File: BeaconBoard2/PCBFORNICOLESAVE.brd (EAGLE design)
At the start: 101.6 x 101.6 mm, 104 parts, among them Q3 FDN340P, U1 ATMega2560, U2 3X3BGA0.4MM

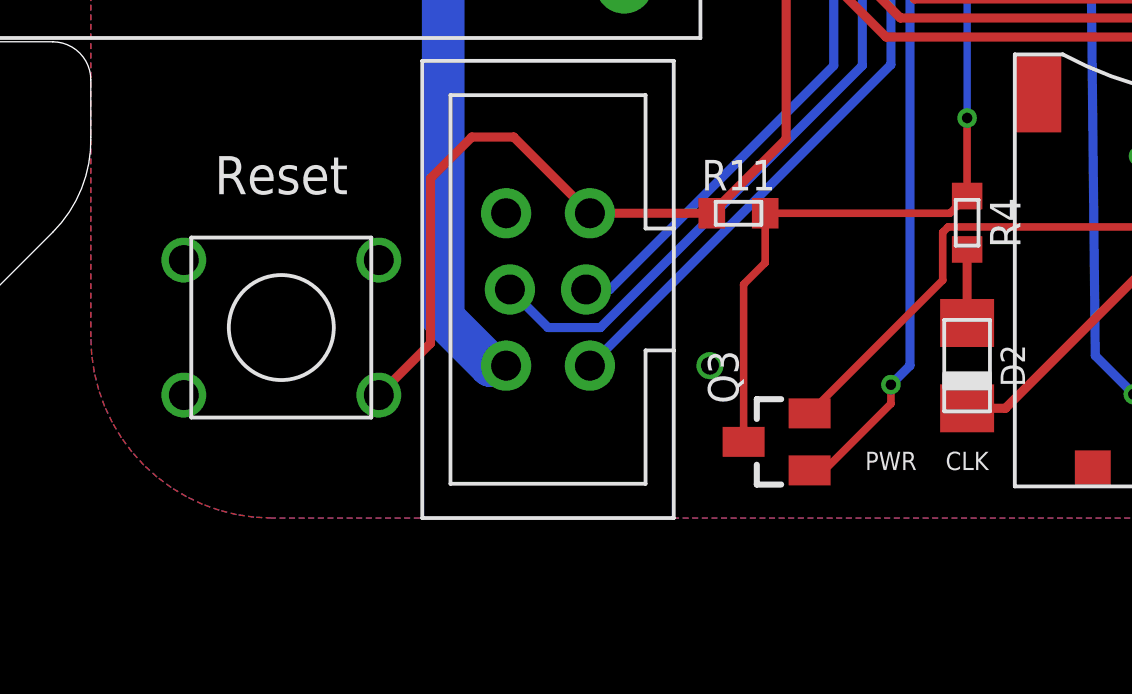
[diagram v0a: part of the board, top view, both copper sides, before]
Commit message: fixed sd card mosfet
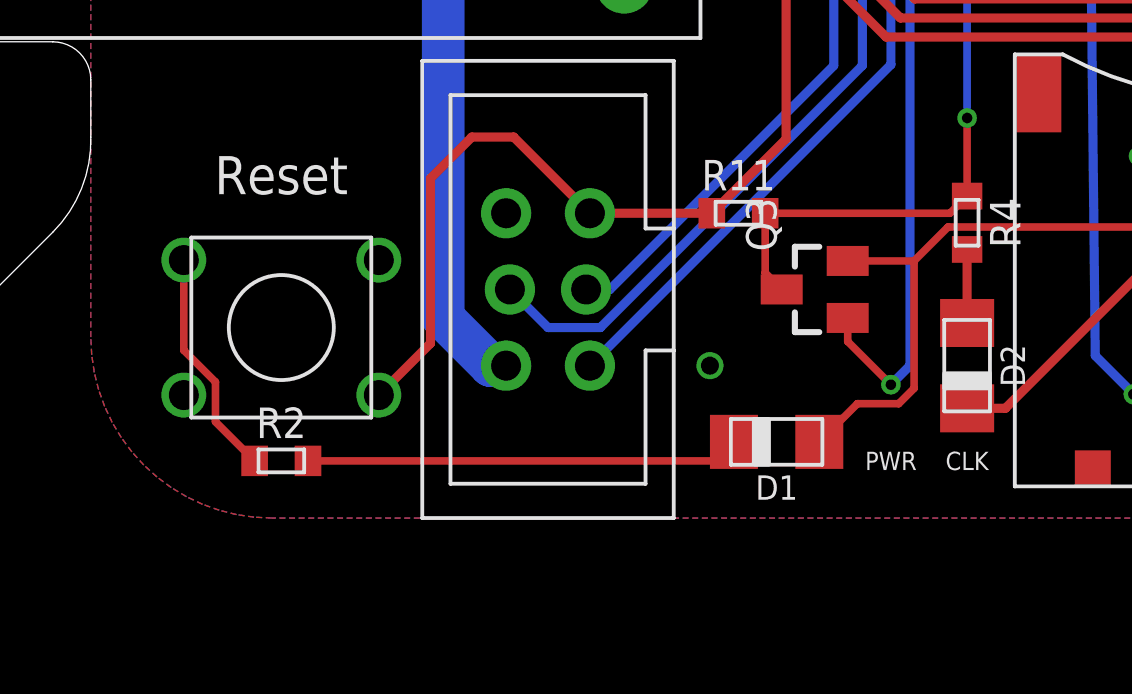
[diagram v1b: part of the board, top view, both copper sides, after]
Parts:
- added D1: (no value), Diodes:1206
- added R2: 1k, Resistors:0603
- moved Q3 5.24 mm to (-14.0, -30.5)
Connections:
- new net N$1: D1.2, R2.2
- net GND: now also R2.1
- net SD_3V3: now also D1.1
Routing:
- net N$1: track 0.00 -> 14.5 mm
- net GND: track 26.4 -> 34.1 mm
- net 3V3: track 298.5 -> 293.3 mm
- net SD_3V3: track 20.8 -> 24.6 mm
- net SD_PWR: track 35.7 -> 34.3 mm
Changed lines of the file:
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@@
 <attribute name="VALUE" x="-23.495" y="31.75" size="1.27" layer="27" rot="R90"/>
 </element>
-<element name="Q3" library="FDN340P" package="SSOT-3" value="FDN340P" x="-15.24" y="-35.56" smashed="yes" rot="R90">
-<attribute name="AVAILABILITY" value="Unavailable" x="-15.24" y="-35.56" size="1.778" layer="27" rot="R90" display="off"/>
-<attribute name="DESCRIPTION" value=" Die Assymertrical For Fdc6329l " x="-15.24" y="-35.56" size="1.778" layer="27" rot="R90" display="off"/>
-<attribute name="MF" value="MICROSS/On Semiconductor" x="-15.24" y="-35.56" size="1.778" layer="27" rot="R90" display="off"/>
-<attribute name="MP" value="FDN340P" x="-15.24" y="-35.56" size="1.778" layer="27" rot="R90" display="off"/>
-<attribute name="NAME" x="-16.510309375" y="-34.289690625" size="1.016240625" layer="25" ratio="18" rot="R90"/>
-<attribute name="PACKAGE" value="TO-236-3 Micross" x="-15.24" y="-35.56" size="1.778" layer="27" rot="R90" display="off"/>
-<attribute name="PRICE" value="None" x="-15.24" y="-35.56" size="1.778" layer="27" rot="R90" display="off"/>
-<attribute name="VALUE" x="-12.058709375" y="-37.46876875" size="0.814409375" layer="27" ratio="10" rot="R90"/>
+<element name="Q3" library="FDN340P" package="SSOT-3" value="FDN340P" x="-13.97" y="-30.48" smashed="yes" rot="R90">
+<attribute name="AVAILABILITY" value="Unavailable" x="-13.97" y="-30.48" size="1.778" layer="27" rot="R90" display="off"/>
+<attribute name="DESCRIPTION" value=" Die Assymertrical For Fdc6329l " x="-13.97" y="-30.48" size="1.778" layer="27" rot="R90" display="off"/>
+<attribute name="MF" value="MICROSS/On Semiconductor" x="-13.97" y="-30.48" size="1.778" layer="27" rot="R90" display="off"/>
+<attribute name="MP" value="FDN340P" x="-13.97" y="-30.48" size="1.778" layer="27" rot="R90" display="off"/>
+<attribute name="NAME" x="-15.240309375" y="-29.209690625" size="1.016240625" layer="25" ratio="18" rot="R90"/>
+<attribute name="PACKAGE" value="TO-236-3 Micross" x="-13.97" y="-30.48" size="1.778" layer="27" rot="R90" display="off"/>
+<attribute name="PRICE" value="None" x="-13.97" y="-30.48" size="1.778" layer="27" rot="R90" display="off"/>
+<attribute name="VALUE" x="-10.788709375" y="-32.38876875" size="0.814409375" layer="27" ratio="10" rot="R90"/>
+</element>
+<element name="D1" library="Diodes" package="1206" value="" x="-15.24" y="-35.56" smashed="yes" rot="R180">
+<attribute name="NAME" x="-15.24" y="-37.084" size="0.8128" layer="25" rot="R180" align="center"/>
+</element>
+<element name="R2" library="Resistors" package="0603" value="1k" x="-31.75" y="-36.195" smashed="yes">
+<attribute name="NAME" x="-31.75" y="-34.925" size="1.016" layer="25" align="center"/>
+<attribute name="VALUE" x="-31.75" y="-37.465" size="1.016" layer="27" align="center"/>
 </element>
 </elements>
@@
 <wire x1="-5.21" y1="-14.2875" x2="-8.7025" y2="-17.78" width="0.254" layer="1"/>
 <wire x1="-8.89" y1="-17.78" x2="-8.7025" y2="-17.78" width="0.254" layer="1"/>
-<wire x1="-16.34" y1="-30.31" x2="-16.34" y2="-35.56" width="0.254" layer="1"/>
-<wire x1="-15.621" y1="-29.591" x2="-16.34" y2="-30.31" width="0.254" layer="1"/>
-<wire x1="-15.621" y1="-29.591" x2="-15.621" y2="-27.94" width="0.254" layer="1"/>
+<wire x1="-15.621" y1="-27.94" x2="-15.621" y2="-29.929" width="0.254" layer="1"/>
+<wire x1="-15.07" y1="-30.48" x2="-15.621" y2="-29.929" width="0.254" layer="1"/>
 <wire x1="-15.621" y1="-27.94" x2="-9.4615" y2="-27.94" width="0.254" layer="1"/>
 <wire x1="8.41375" y1="-7.77875" x2="6.0325" y2="-5.3975" width="1.651" layer="16"/>
@@
 <via x="2.54" y="-26.035" extent="1-16" drill="0.35"/>
 <wire x1="-3.175" y1="-26.035" x2="2.54" y2="-26.035" width="0.254" layer="16"/>
+<contactref element="R2" pad="1"/>
+<wire x1="-35" y1="-29.5" x2="-35" y2="-32.5082875" width="0.254" layer="1"/>
+<wire x1="-33.9452" y1="-34.8888" x2="-32.639" y2="-36.195" width="0.254" layer="1"/>
+<wire x1="-35" y1="-32.5082875" x2="-33.9452" y2="-33.5630875" width="0.254" layer="1"/>
+<wire x1="-33.9452" y1="-33.5630875" x2="-33.9452" y2="-34.8888" width="0.254" layer="1"/>
 </signal>
 <signal name="BT_TX">
@@
 <wire x1="-10.795" y1="-33.02" x2="-11.43" y2="-33.655" width="0.3048" layer="16"/>
 <via x="-11.43" y="-33.655" extent="1-16" drill="0.35"/>
-<wire x1="-11.43" y1="-33.655" x2="-11.43" y2="-34.29" width="0.254" layer="1"/>
-<wire x1="-11.43" y1="-34.29" x2="-13.65" y2="-36.51" width="0.254" layer="1"/>
-<wire x1="-14.14" y1="-36.51" x2="-13.65" y2="-36.51" width="0.254" layer="1"/>
+<wire x1="-12.87" y1="-31.43" x2="-12.87" y2="-32.215" width="0.254" layer="1"/>
+<wire x1="-11.43" y1="-33.655" x2="-12.87" y2="-32.215" width="0.254" layer="1"/>
 </signal>
 <signal name="SD_CD">
@@
 <contactref element="Q3" pad="2"/>
 <wire x1="-9.52425" y1="-28.3972" x2="-2.9972" y2="-28.3972" width="0.254" layer="1"/>
-<wire x1="-9.7028" y1="-28.57575" x2="-9.52425" y2="-28.3972" width="0.254" layer="1"/>
-<wire x1="-14.14" y1="-34.61" x2="-9.7028" y2="-30.1728" width="0.254" layer="1"/>
-<wire x1="-9.7028" y1="-30.1728" x2="-9.7028" y2="-28.57575" width="0.254" layer="1"/>
+<wire x1="-9.52425" y1="-28.3972" x2="-10.65705" y2="-29.53" width="0.254" layer="1"/>
+<wire x1="-12.87" y1="-29.53" x2="-10.65705" y2="-29.53" width="0.254" layer="1"/>
 <wire x1="-2.9972" y1="-28.3972" x2="0.3" y2="-25.1" width="0.254" layer="1"/>
 <wire x1="0.3" y1="-25.1" x2="0.3" y2="-23.645" width="0.254" layer="1"/>
+<contactref element="D1" pad="1"/>
+<wire x1="-13.818" y1="-35.56" x2="-12.5452" y2="-34.2872" width="0.254" layer="1"/>
+<wire x1="-12.5452" y1="-34.2872" x2="-11.16813125" y2="-34.2872" width="0.254" layer="1"/>
+<wire x1="-11.16813125" y1="-34.2872" x2="-10.65705" y2="-33.77611875" width="0.254" layer="1"/>
+<wire x1="-10.65705" y1="-33.77611875" x2="-10.65705" y2="-29.53" width="0.254" layer="1"/>
+</signal>
+<signal name="N$1">
+<contactref element="D1" pad="2"/>
+<contactref element="R2" pad="2"/>
+<wire x1="-30.861" y1="-36.195" x2="-17.297" y2="-36.195" width="0.254" layer="1"/>
+<wire x1="-17.297" y1="-36.195" x2="-16.662" y2="-35.56" width="0.254" layer="1"/>
 </signal>
 </signals>
